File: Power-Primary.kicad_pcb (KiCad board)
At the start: 2 copper layers, 226.1 x 72.4 mm, 77 parts, among them J1 HV in, J10 SPARE, J11 SPARE, J12 SPARE, J13 SPARE, J14 SPARE, J15 SPARE, J16 SPARE, J17 SPARE, J2 Dashboard, J3 Telemetry, J4 Motor, J5 MPPT 1, J6 MPPT 2, J7 BPS, J8 Primary Disconn., J9 SPARE, U1 Mean_Well_12V

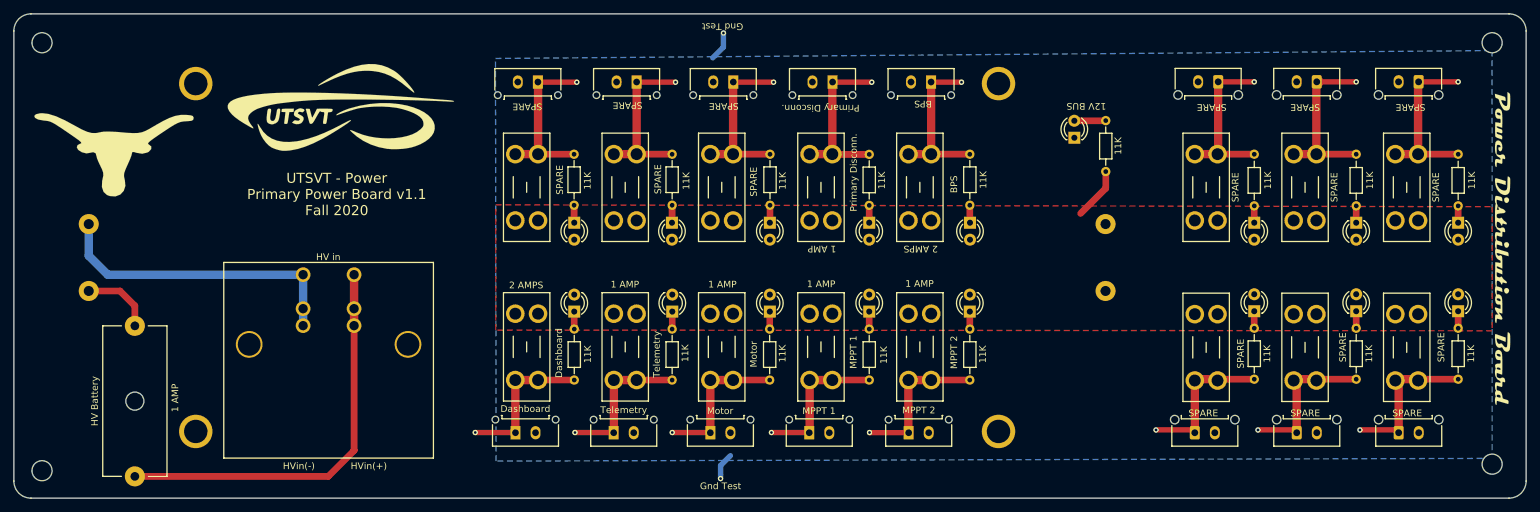
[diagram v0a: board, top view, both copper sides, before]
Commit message: completed Hannah's edits
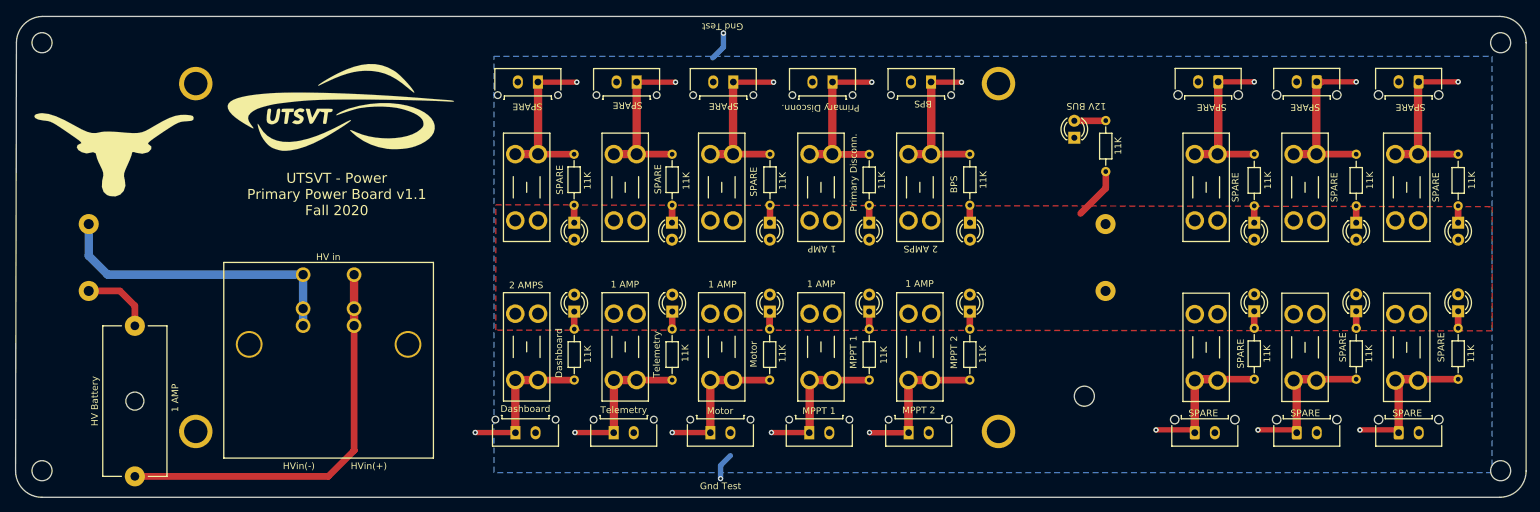
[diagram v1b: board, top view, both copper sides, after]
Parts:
- removed the G*** at (226.1, 104.1)
- added REF**: MountingHole_3mm, MountingHole:MountingHole_3.7mm, F.Cu at (175.3, 113.0)
- moved REF** 1.60 mm to (237.5, 124.2)
- moved REF** 1.27 mm to (237.5, 60.2)
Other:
- board size 226.1 x 72.4 mm -> 225.8 x 71.9 mm
